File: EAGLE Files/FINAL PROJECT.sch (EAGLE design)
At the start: 18 parts, among them J1 BATTERY, U1 9_to_3.3_VREG

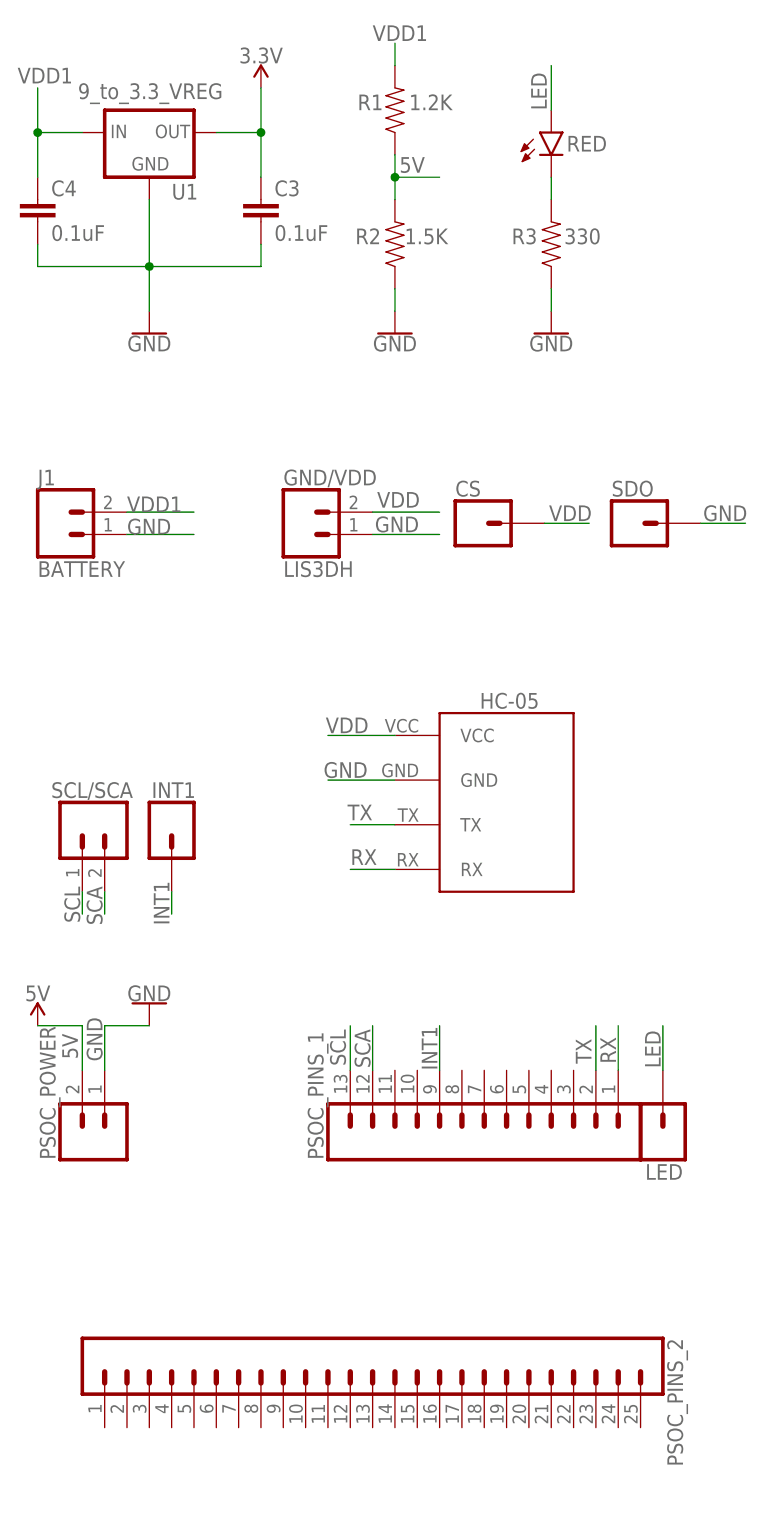
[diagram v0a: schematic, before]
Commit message: final EAGLE files
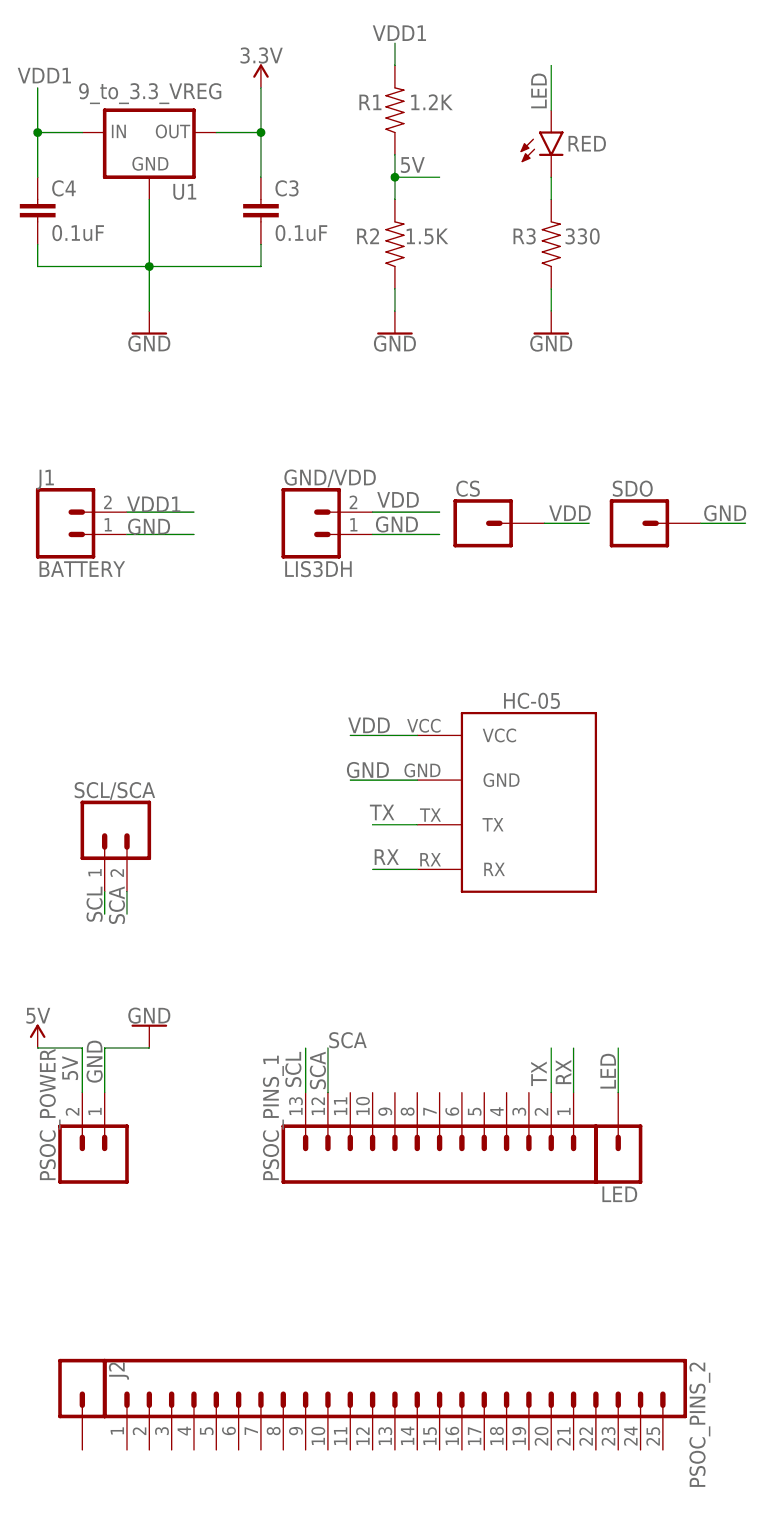
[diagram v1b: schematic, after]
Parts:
- removed INT1: (no value), SparkFun-Connectors:CONN_01
- added J2: (no value), SparkFun-Connectors:CONN_01
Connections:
- removed net INT1: INT1.1, PSOC_PINS_1.9
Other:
- moved on the sheet: HC-05, LED, PSOC_PINS_1, PSOC_PINS_2, PSOC_POWER, SCL/SCA
